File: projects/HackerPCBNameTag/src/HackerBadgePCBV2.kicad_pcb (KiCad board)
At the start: 2 copper layers, 88 x 115.6 mm, 31 parts, among them Q1 S8050, Q2 FS8205, U1 NT3H2111W0FHKH, U2 TPS61023DRLR, U3 DW01A_C351410

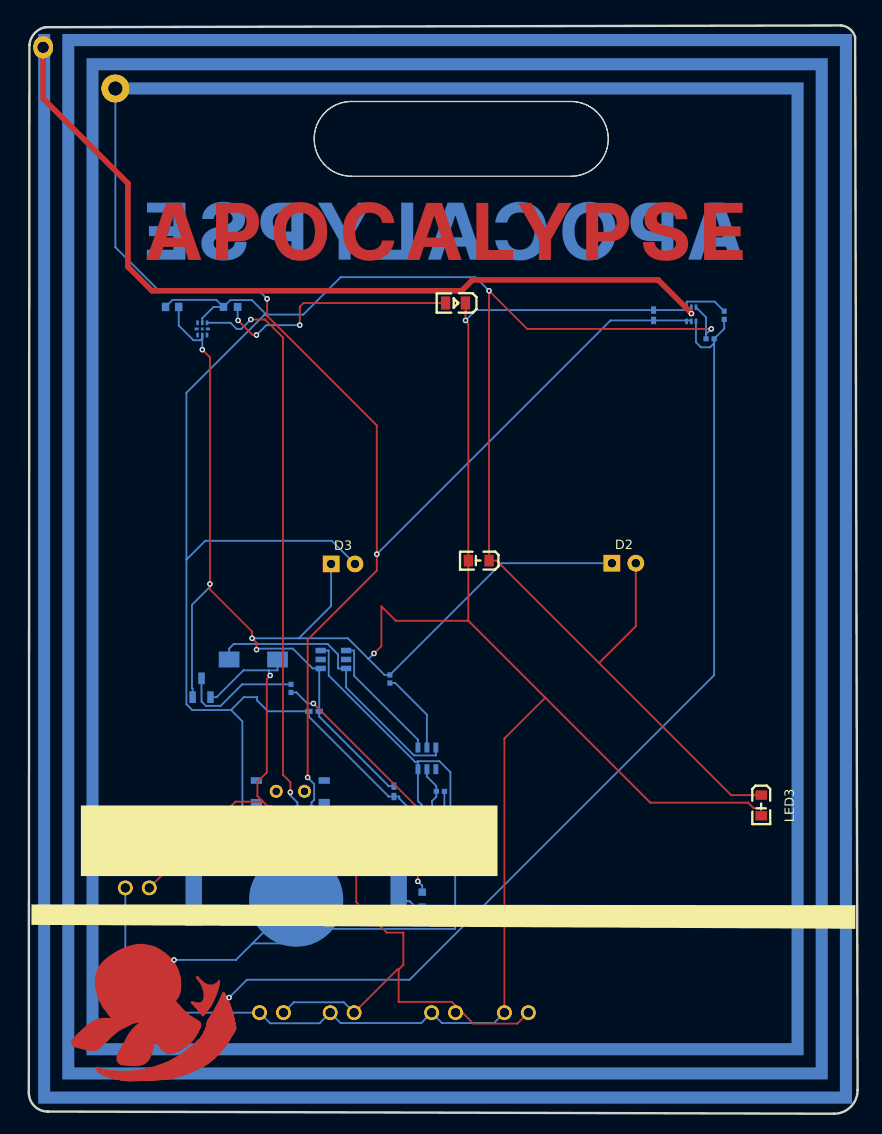
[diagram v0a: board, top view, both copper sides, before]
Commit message: some updates
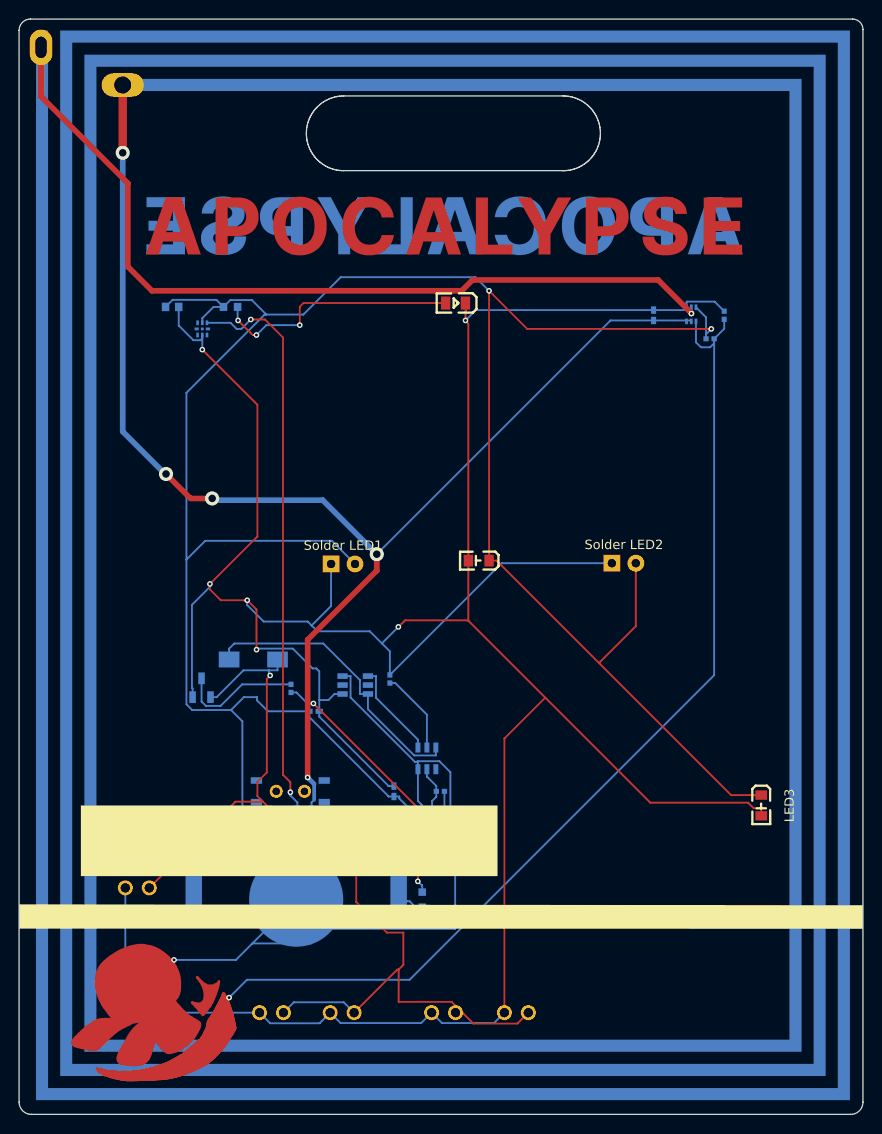
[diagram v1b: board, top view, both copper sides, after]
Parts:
- removed Q2: FS8205, easyeda2kicad:SOT-23-6_L2.9-W1.6-P0.95-LS2.8-BR
- added Q3: FS8205A, easyeda2kicad:SOT-23-6_L2.9-W1.6-P0.95-LS2.8-BR, B.Cu at (126.4, 114.7)
- Solder LED1: renamed from D3
- Solder LED2: renamed from D2
- moved L1 0.43 mm to (135.7, 102.0)
- renumbered SWITCH1 to ON/OFF
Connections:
- L1 pad 3: (no net) -> Net-(U2-EN)
- ON/OFF pad 4: unconnected-(SWITCH1-Pad4)_1 -> /unconnected-(SWITCH1-Pad4)_1_1_1_1
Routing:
- net GND: track 340.9 -> 344.8 mm
- net Net-(Q3-G2): track 14.0 -> 10.3 mm
- net BAT-: track 80.8 -> 77.1 mm
- net Net-(U2-EN): track 141.9 -> 145.4 mm, vias 3 -> 5
- net VCC: track 294.1 -> 293.4 mm
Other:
- board size 88 x 115.6 mm -> 89.6 x 116.3 mm
